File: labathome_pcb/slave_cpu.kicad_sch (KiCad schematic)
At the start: 32 parts, among them J27 ADDA, J34 STM32 EXT, J36 PROG_STM, U16 LM358, U5 STM32G431R8Tx

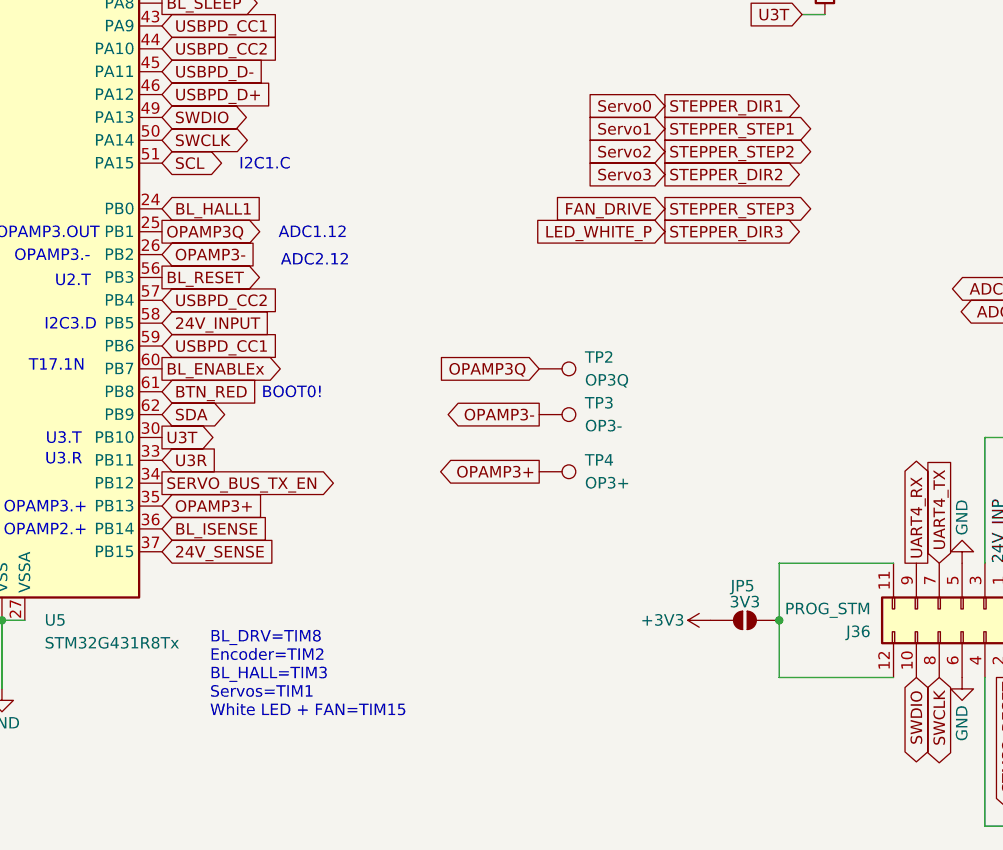
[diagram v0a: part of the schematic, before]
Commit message: Merged
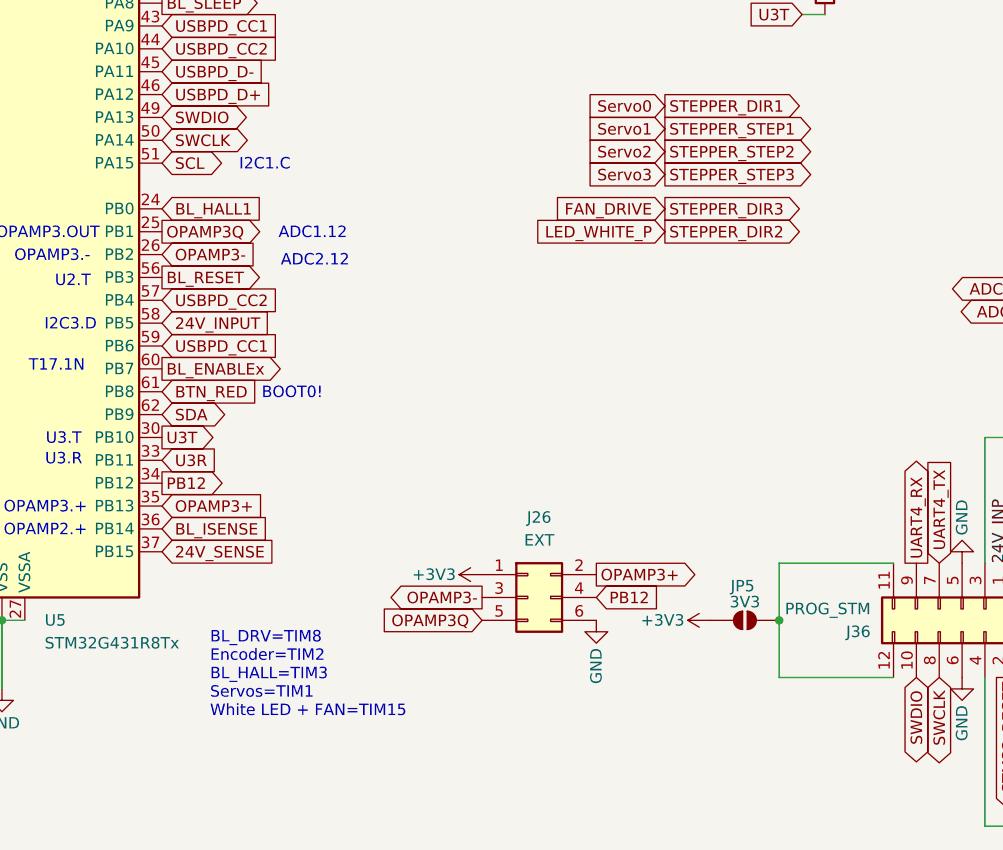
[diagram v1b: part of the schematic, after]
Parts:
- removed TP2: OP3Q, TestPoint:TestPoint_Pad_1.5x1.5mm, symbol Connector:TestPoint
- removed TP3: OP3-, TestPoint:TestPoint_Pad_1.5x1.5mm, symbol Connector:TestPoint
- removed TP4: OP3+, TestPoint:TestPoint_Pad_1.5x1.5mm, symbol Connector:TestPoint
- added J26: EXT, Connector_PinHeader_2.54mm:PinHeader_2x03_P2.54mm_Vertical, symbol Connector_Generic:Conn_02x03_Odd_Even
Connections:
- net SERVO_BUS_TX_EN is gone; now on net PB12: U5.34 (PB12)
- net +3V3: now also J26.1 (Pin_1)
- net GND: now also J26.6 (Pin_6)
- net OPAMP3+: now also J26.2 (Pin_2)
- net OPAMP3-: now also J26.3 (Pin_3)
- net OPAMP3Q: now also J26.5 (Pin_5)
- net PB12: now also J26.4 (Pin_4)
- net STEPPER_DIR2 renamed STEPPER_STEP3
